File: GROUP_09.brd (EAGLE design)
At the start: 160 x 100 mm, 29 parts, among them J1 POWER_JACKPTH_LOCK, U1 +12v, U3 TCA9546ATSSOP16, U4 TMUX1208QNF

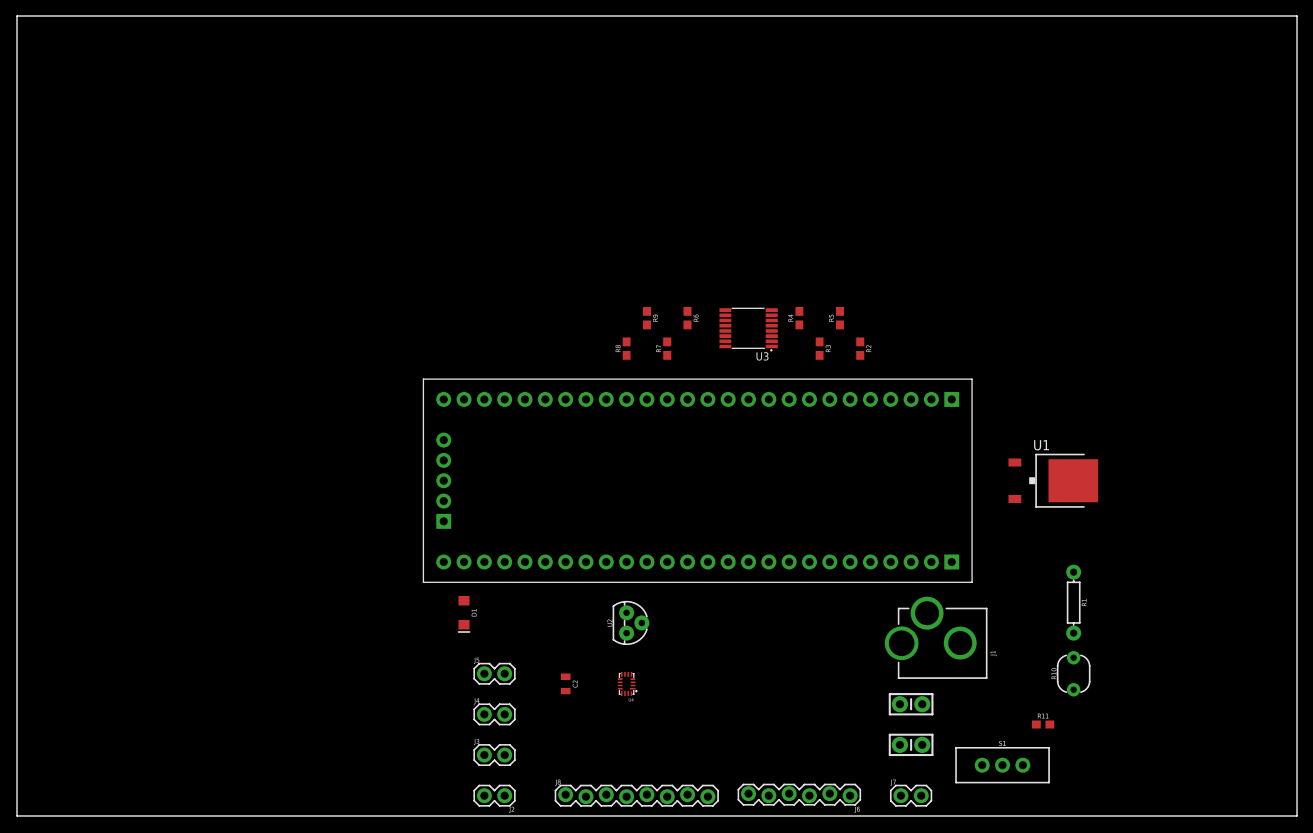
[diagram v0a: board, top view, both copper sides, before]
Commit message: board V1.01
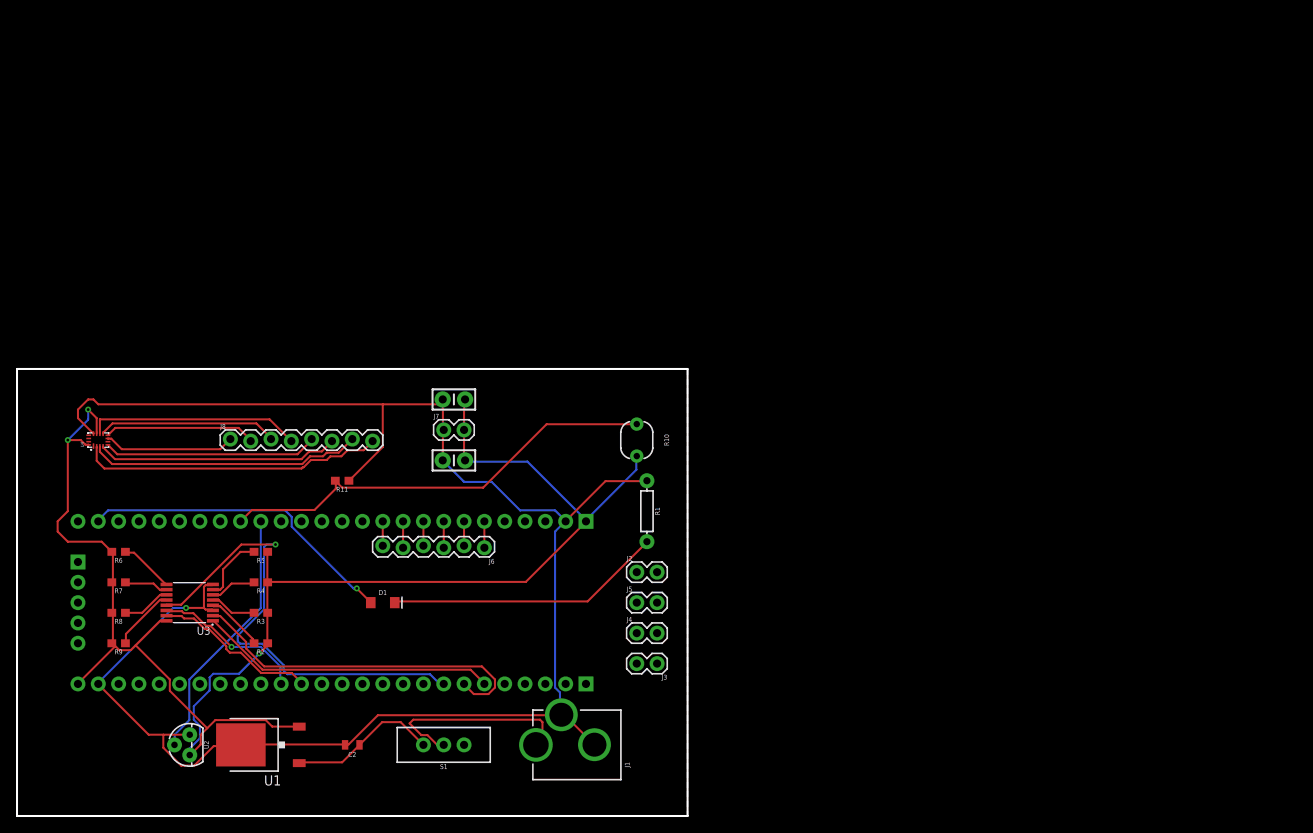
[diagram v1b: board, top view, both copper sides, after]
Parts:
- moved U1 104.4 mm to (30.5, 8.89), turned to 90 degrees
- moved R11 92.8 mm to (40.6, 41.9), turned to 180 degrees
- moved R2 83.5 mm to (30.5, 21.6), turned to 180 degrees
- moved R5 78.1 mm to (30.5, 33.0), turned to 180 degrees
- moved U3 77.8 mm to (21.6, 26.7)
- moved R9 77.5 mm to (12.7, 21.6), turned to 180 degrees
- moved R3 77.3 mm to (30.5, 25.4), turned to 180 degrees
- moved R6 76.9 mm to (12.7, 33.0), turned to 180 degrees
- moved R4 75.0 mm to (30.5, 29.2), turned to 180 degrees
- moved R7 74.5 mm to (12.7, 29.2), turned to 180 degrees
- moved J7 73.2 mm to (53.3, 48.3)
- moved U4 72.7 mm to (10.2, 47.0), turned to 90 degrees
- moved R8 71.6 mm to (12.7, 25.4), turned to 180 degrees
- moved S1 69.9 mm to (53.3, 8.89), turned to 90 degrees
- moved C3 68.7 mm to (54.6, 52.1)
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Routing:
- net GND: track 0.00 -> 222.6 mm, vias 0 -> 1
- net 5V: track 0.00 -> 202.2 mm, vias 0 -> 3
- net I2C_A2: track 0.00 -> 60.0 mm, vias 0 -> 1
- net PHOTO_OUT: track 0.00 -> 56.2 mm
- net I2C_A1: track 0.00 -> 44.8 mm
- net N$6: track 0.00 -> 40.2 mm, vias 0 -> 1
- net N$25: track 0.00 -> 38.1 mm
- net I2C_A0: track 0.00 -> 37.2 mm
- net N$11: track 0.00 -> 34.7 mm
- net N$24: track 0.00 -> 34.3 mm
- net TEMP_OUT: track 0.00 -> 32.4 mm
- net N$23: track 0.00 -> 30.3 mm
- net N$21: track 0.00 -> 26.8 mm
- net N$22: track 0.00 -> 26.8 mm
- net N$2: track 0.00 -> 26.0 mm
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- added copper zone on layer 1, net 5V
- added copper zone on layer 16, net GND
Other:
- board size 160 x 100 mm -> 83.8 x 55.9 mm
